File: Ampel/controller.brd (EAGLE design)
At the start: 100 x 80 mm, 14 parts, among them IC1 ATtiny25, IC2 7805L, X1 22-23-2041, X2 KUSBVX

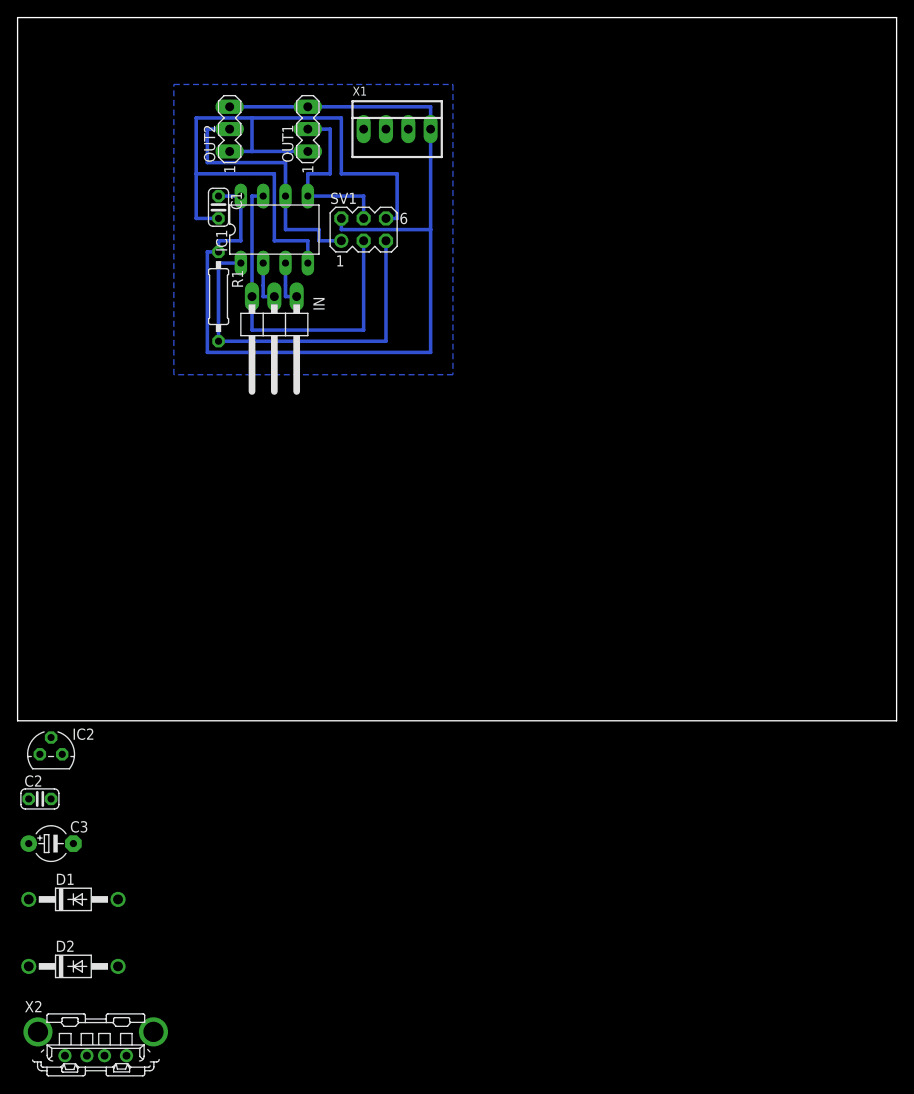
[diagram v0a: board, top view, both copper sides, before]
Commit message: some routing
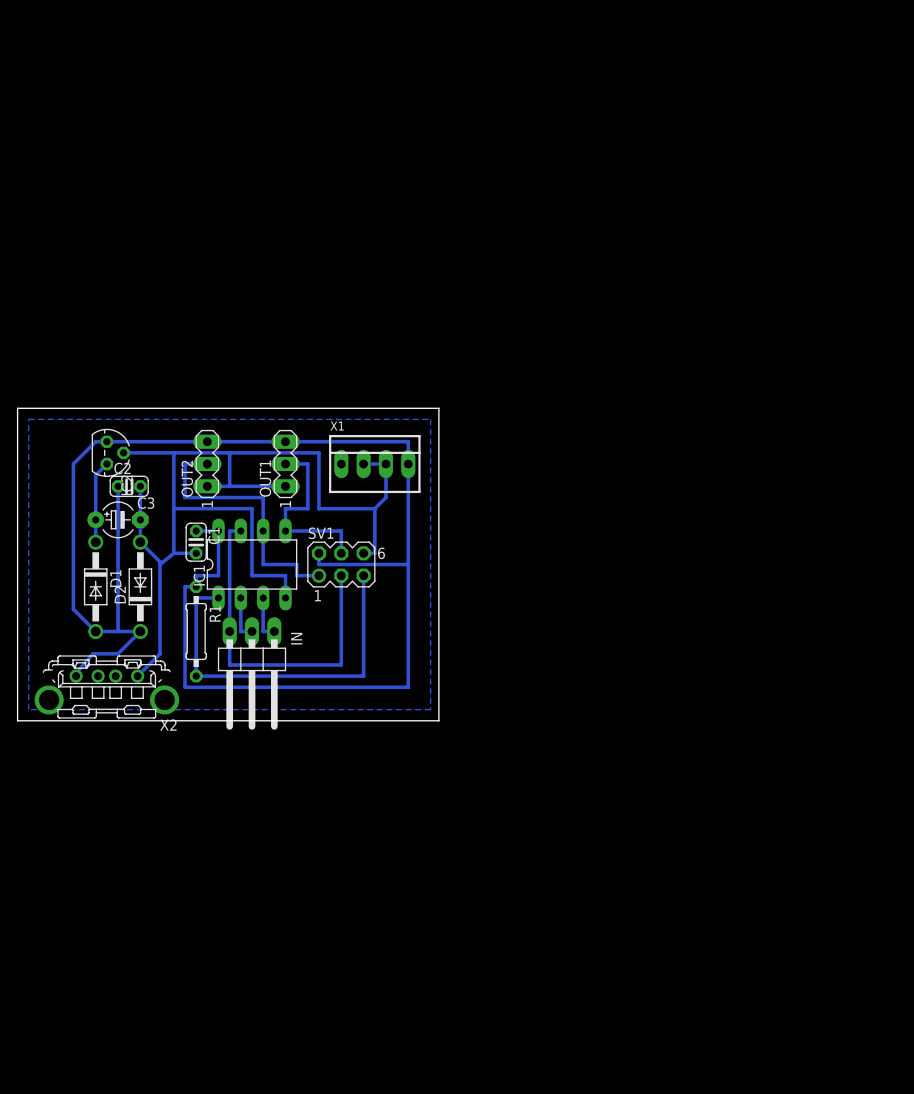
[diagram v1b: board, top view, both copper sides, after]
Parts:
- moved D2 43.8 mm to (14.0, 15.2), turned to 90 degrees
- moved X2 43.2 mm to (10.2, 5.08), turned to 180 degrees
- moved C1 38.2 mm to (20.3, 20.3)
- moved IC1 38.2 mm to (26.7, 17.8)
- moved IN 38.2 mm to (26.7, 6.35)
- moved OUT1 38.2 mm to (30.5, 29.2)
- moved OUT2 38.2 mm to (21.6, 29.2)
- moved SV1 38.2 mm to (36.8, 17.8)
- moved X1 38.2 mm to (40.6, 29.2)
- moved R1 38.2 mm to (20.3, 10.2)
- moved C3 37.6 mm to (11.4, 22.9)
- moved C2 37.0 mm to (12.7, 26.7)
- moved D1 35.7 mm to (8.89, 15.2), turned to 270 degrees
- moved IC2 34.9 mm to (10.2, 30.5), turned to 270 degrees
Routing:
- net VCC: track 111.8 -> 179.4 mm
- net GND: track 85.1 -> 124.5 mm
- net VEE: track 0.00 -> 9.42 mm
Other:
- board size 100 x 80 mm -> 47.9 x 35.5 mm
